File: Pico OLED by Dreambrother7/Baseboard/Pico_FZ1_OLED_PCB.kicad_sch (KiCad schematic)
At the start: 17 parts, among them J1 SSD1309 OLED, J2 2x5 Header, U1 Pico

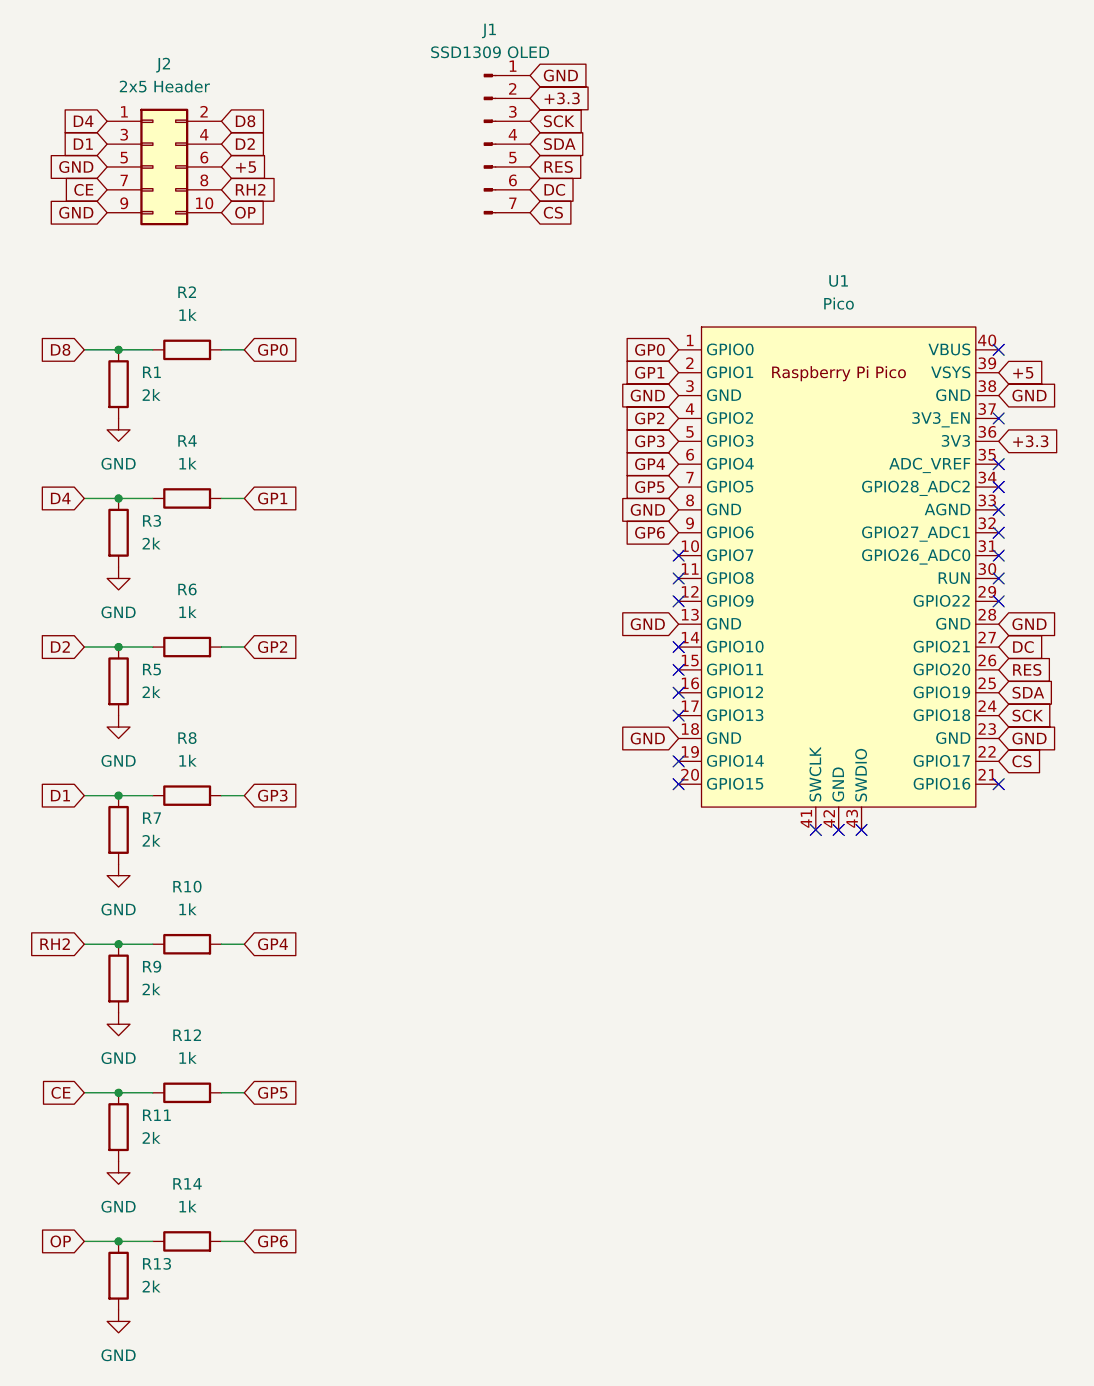
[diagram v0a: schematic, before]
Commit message: new PCB design updates
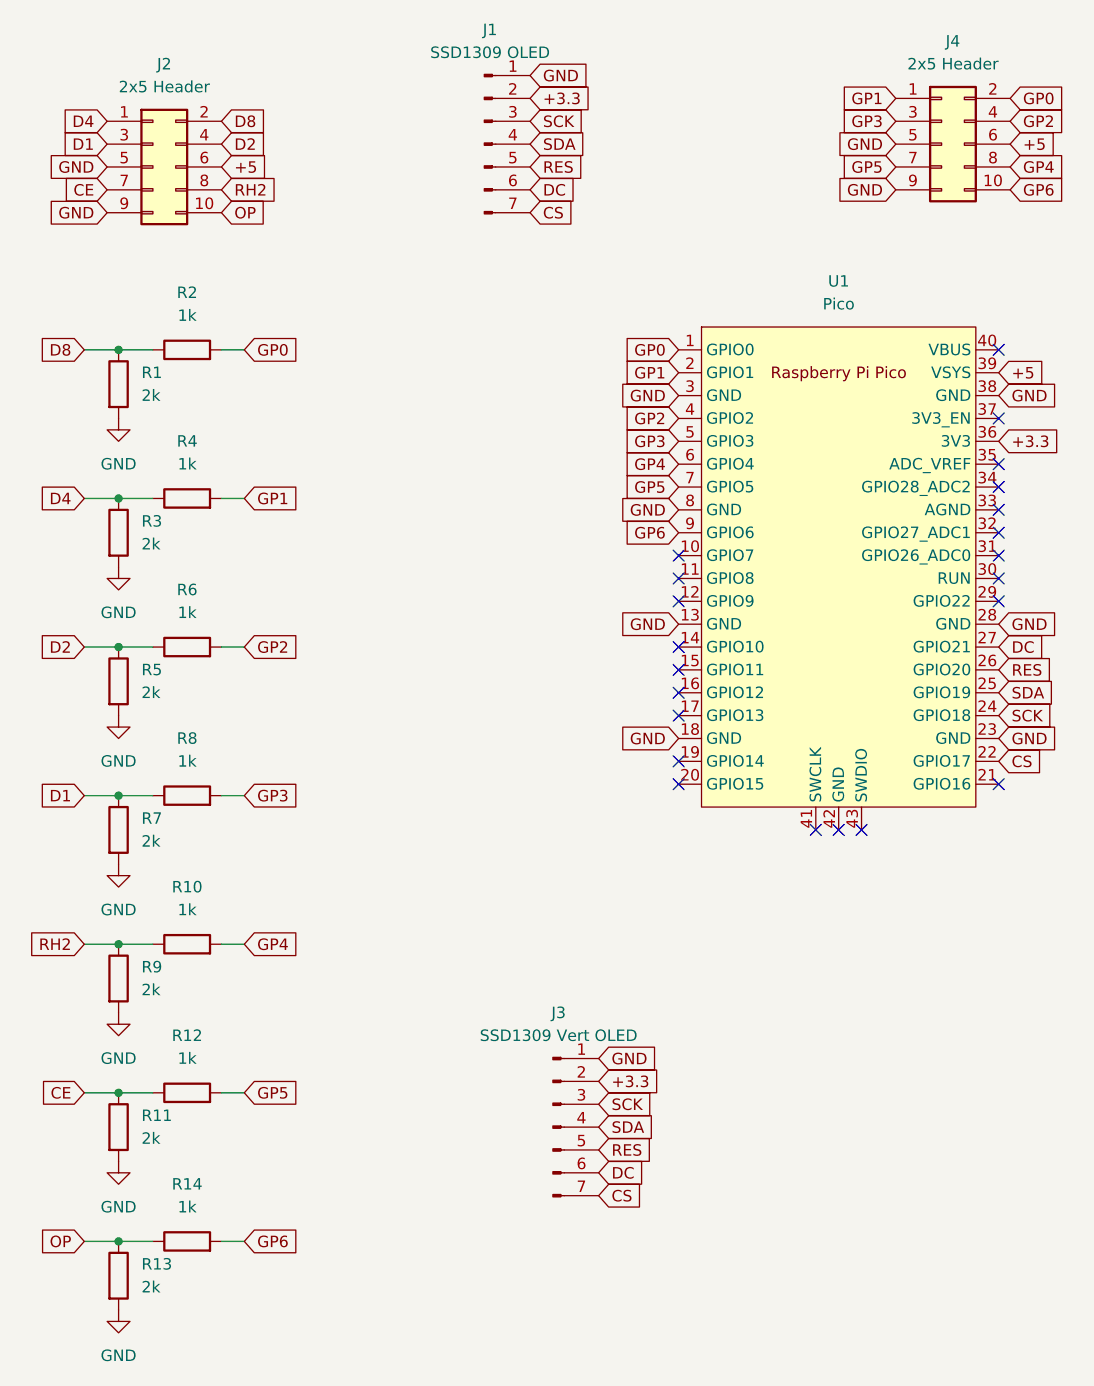
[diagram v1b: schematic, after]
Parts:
- added J3: SSD1309 Vert OLED, Connector_PinHeader_2.54mm:PinHeader_1x07_P2.54mm_Vertical, symbol Connector:Conn_01x07_Pin
- added J4: 2x5 Header, Connector_PinHeader_2.00mm:PinHeader_2x05_P2.00mm_Vertical, symbol Connector_Generic:Conn_02x05_Odd_Even
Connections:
- net +3.3: now also J3.2 (Pin_2)
- net +5: now also J4.6 (Pin_6)
- net CS: now also J3.7 (Pin_7)
- net DC: now also J3.6 (Pin_6)
- net GND: now also J3.1 (Pin_1), J4.5 (Pin_5), J4.9 (Pin_9)
- net GP0: now also J4.2 (Pin_2)
- net GP1: now also J4.1 (Pin_1)
- net GP2: now also J4.4 (Pin_4)
- net GP3: now also J4.3 (Pin_3)
- net GP4: now also J4.8 (Pin_8)
- net GP5: now also J4.7 (Pin_7)
- net GP6: now also J4.10 (Pin_10)
- net RES: now also J3.5 (Pin_5)
- net SCK: now also J3.3 (Pin_3)
- net SDA: now also J3.4 (Pin_4)
